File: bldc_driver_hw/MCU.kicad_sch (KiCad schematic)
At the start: 34 parts, among them SW1 SW_Push, U5 MCP1501-33xSN, U6 STM32G474RETx, Y1 24MHz

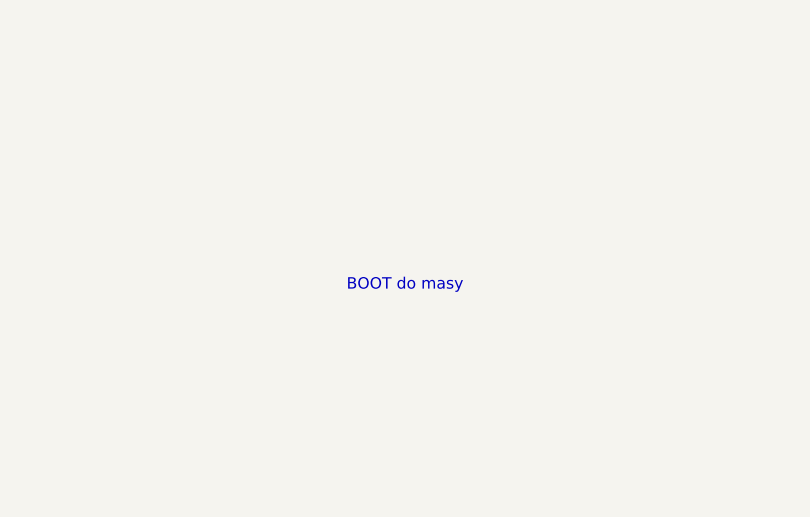
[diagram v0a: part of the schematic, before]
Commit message: wip
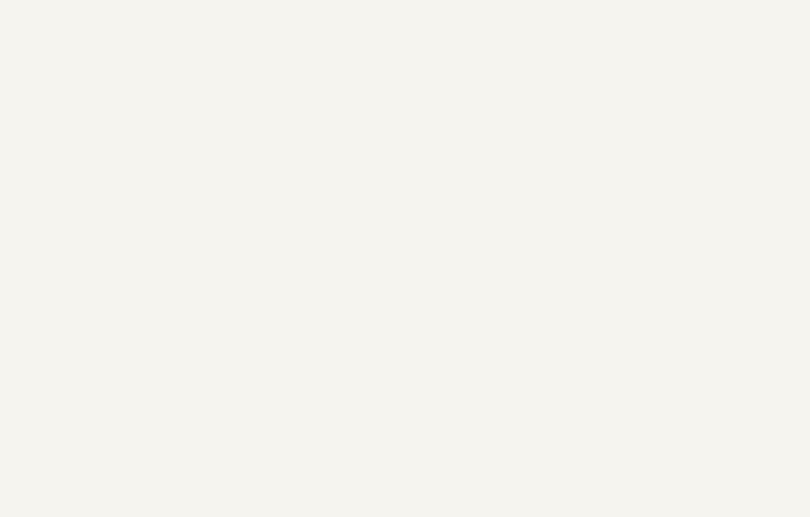
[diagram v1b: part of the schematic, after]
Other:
- note removed: "BOOT do masy"
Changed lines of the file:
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@@
 	(generator_version "9.0")
 	(paper "A4")
-	(text "BOOT do masy\n"
-		(exclude_from_sim no)
-		(at 61.214 140.716 0)
-		(effects
-			(font
-				(size 1.27 1.27)
-			)
-		)
-	)
 	(junction
 		(at 180.34 154.94)

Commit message: wip
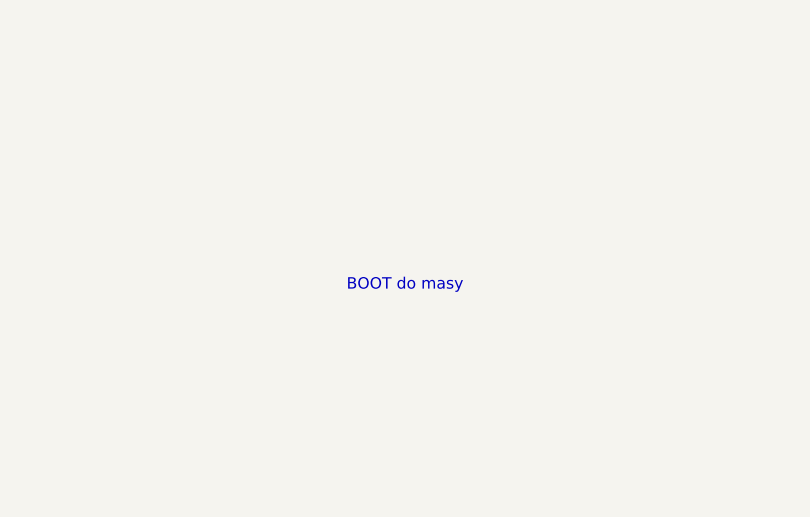
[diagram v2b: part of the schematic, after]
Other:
- note added: "BOOT do masy"
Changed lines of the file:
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@@
 	(generator_version "9.0")
 	(paper "A4")
+	(text "BOOT do masy\n"
+		(exclude_from_sim no)
+		(at 61.214 140.716 0)
+		(effects
+			(font
+				(size 1.27 1.27)
+			)
+		)
+	)
 	(junction
 		(at 180.34 154.94)
